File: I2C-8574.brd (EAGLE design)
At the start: 106 x 100 mm, 89 parts, among them J1 CONNECTOR-I2CLEFT, J11 RJ12/6, J2 CONNECTOR-I2CLEFT, J5 CONNECTOR-GROVE-4P-2.0-347013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, J6 RJ12/6, J7 RJ12/6, J8 CONNECTOR-GROVE-4P-2.0-347013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, J9 RJ12/6, U1 PCF8574DW, U2 PCF8574ADW

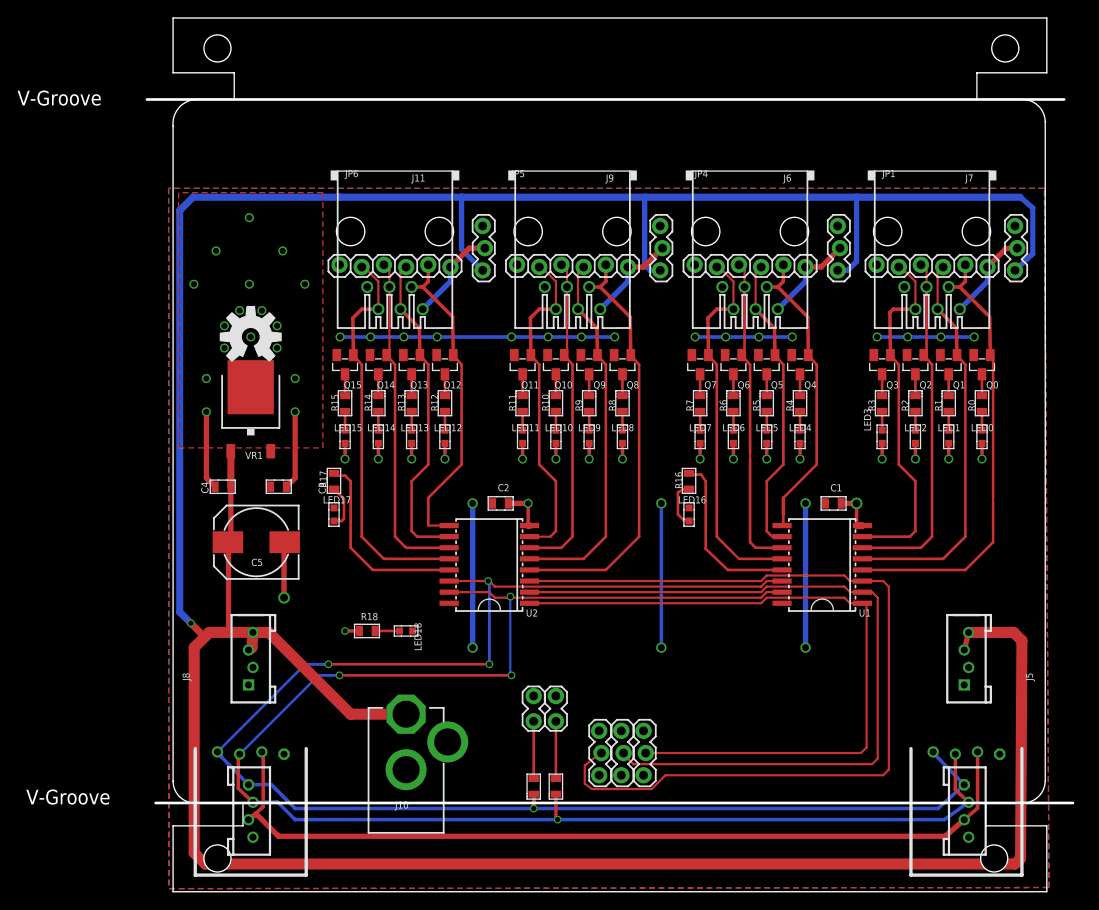
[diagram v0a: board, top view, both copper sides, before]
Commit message: 3.0
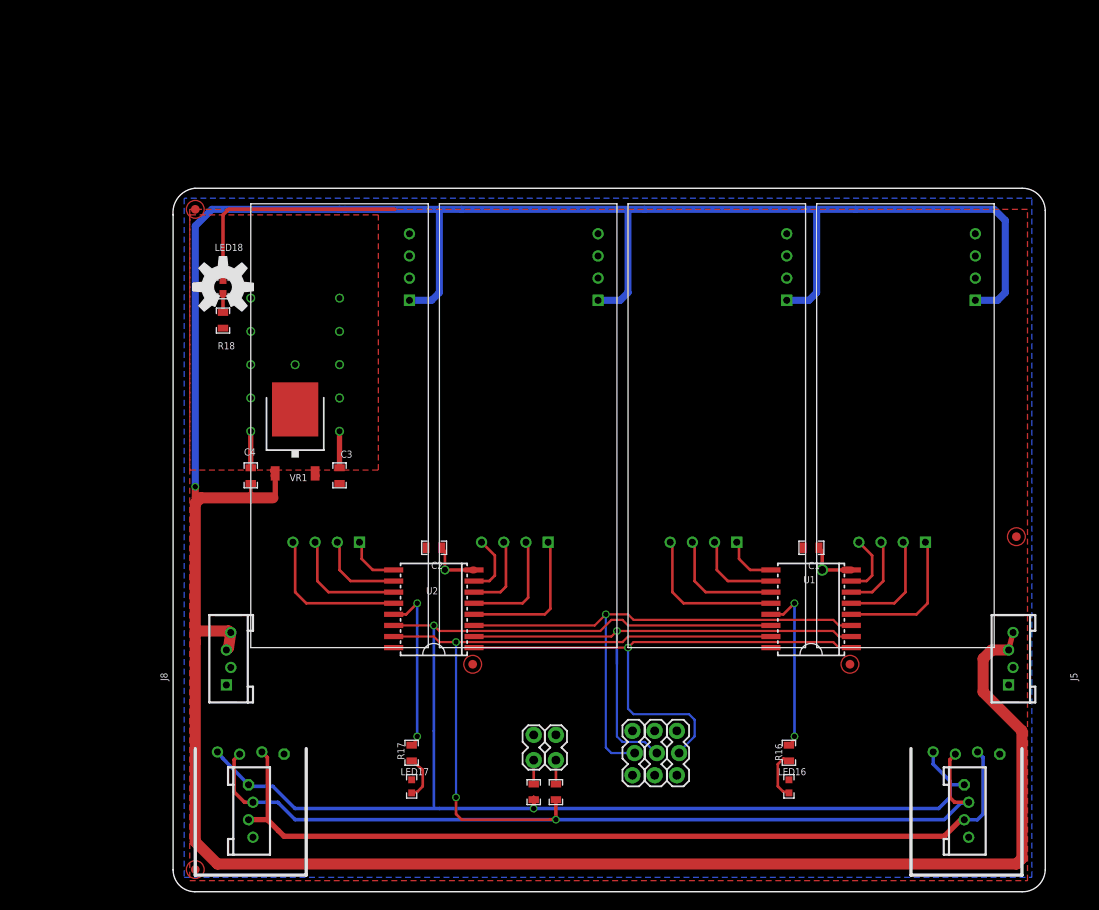
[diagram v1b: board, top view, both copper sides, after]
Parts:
- removed C5: 150uF, SPCoast:0810-CAP
- removed J10: (no value), SPCoast:DCJ0202
- removed J11, J6, J7, J9: RJ12/6, SPCoast:RJ25-PANEL
- removed JP1, JP4, JP5, JP6: .100x1x6, SPCoast:1X06_LOCK
- removed LED0, LED1, LED10, LED11, LED12, LED13, LED14, LED15, LED2, LED3, LED4, LED5, LED6, LED7, LED8, LED9: Y-0330050P1, SPCoast:0603-LED
- removed POWER: 7-12vDC, SPCoast-minimal:POWER_USAGE
- removed Q0, Q1, Q10, Q11, Q12, Q13, Q14, Q15, Q2, Q3, Q4, Q5, Q6, Q7, Q8, Q9: (no value), SPCoast:SOT23
- removed R0, R1, R10, R11, R12, R13, R14, R2, R3, R4, R5, R6, R7, R8, R9: 2K2, SPCoast:0805-RES
- removed R15: 2K0, SPCoast:0805-RES
- removed VIO1, VIO2, VIO3, VIO4: jumper, SPCoast:1X03
- added FID-U1, FID-U2, FID1, FID2, FID3: FIDUCIAL, SPCoast:FIDUCIAL_1MM
- added U$2, U$3, U$4, U$5: IO4-IOBBARE, SPCoast:IO4-IOB
- A1, A2, A3: device SPCoast:1X03 -> SPCoast-minimal:1X03
- BOARD1: value BOARD80X100-NOHOLES -> (none)
- C1, C2, C3, C4: device SPCoast:0805-CAP -> SPCoast-minimal:0805-CAP
- R16, R17, R18: device SPCoast:0805-RES -> SPCoast-minimal:0805-RES
- SCL, SDA: device SPCoast:1X02_LOCK -> SPCoast-minimal:1X02_LOCK
- U1, U2: device SPCoast:SO-16DW -> SPCoast-minimal:SO-16DW
- moved LED18 44.6 mm to (5.71, 69.2), turned to 270 degrees
- moved R18 39.2 mm to (5.71, 65.4), turned to 270 degrees
- moved LED16 33.1 mm to (70.5, 12.1)
- moved R16 33.1 mm to (70.5, 15.9)
- moved LED17 32.4 mm to (27.3, 12.1)
- moved R17 32.4 mm to (27.3, 15.9)
- moved C2 9.16 mm to (29.8, 39.4)
- moved U2 8.13 mm to (29.8, 32.4)
- moved C3 7.10 mm to (19.1, 47.6), turned to 90 degrees
- moved U$1 6.54 mm to (5.71, 69.2)
- moved C1 5.68 mm to (73.0, 39.4)
- moved VR1 5.68 mm to (14.0, 52.7)
- moved U1 5.24 mm to (73.0, 32.4)
- moved J5 5.08 mm to (95.9, 26.7)
- moved SCL 4.44 mm to (43.8, 15.2)
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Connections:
- removed net N$10: LED7.A, R7.1
- removed net N$11: Q0.3, R0.2
- removed net N$12: Q5.3, R5.2
- removed net N$13: Q6.3, R6.2
- removed net N$14: Q7.3, R7.2
- removed net N$15: LED8.A, R8.1
- removed net N$16: LED9.A, R9.1
- removed net N$17: LED10.A, R10.1
- removed net N$18: Q8.3, R8.2
- removed net N$2: LED0.A, R0.1
- removed net N$22: Q9.3, R9.2
- removed net N$23: Q10.3, R10.2
- removed net N$24: Q11.3, R11.2
- removed net N$25: LED11.A, R11.1
- removed net N$26: LED14.A, R14.1
- removed net N$27: LED12.A, R12.1
- removed net N$28: LED13.A, R13.1
- removed net N$29: LED15.A, R15.1
- removed net N$3: LED1.A, R1.1
- removed net N$30: Q1.3, R1.2
- removed net N$31: Q2.3, R2.2
- removed net N$32: Q3.3, R3.2
- removed net N$33: Q12.3, R12.2
- removed net N$34: Q13.3, R13.2
- removed net N$35: Q14.3, R14.2
- removed net N$36: Q15.3, R15.2
- removed net N$4: LED2.A, R2.1
- removed net N$5: LED3.A, R3.1
- removed net N$6: LED4.A, R4.1
- removed net N$7: LED5.A, R5.1
- removed net N$8: Q4.3, R4.2
- removed net N$9: LED6.A, R6.1
- removed net VCC-IO1: J7.1, JP1.6, VIO1.2
- removed net VCC-IO2: J6.1, JP4.6, VIO2.2
- removed net VCC-IO3: J9.1, JP5.6, VIO3.2
- removed net VCC-IO4: J11.1, JP6.6, VIO4.2
- net +9V: now also U$2.V+, U$3.V+, U$4.V+, U$5.V+; no longer C5.+, J10.1, VIO1.3, VIO2.3, VIO3.3, VIO4.3
- net GND: now also U$2.G@1, U$2.G@2, U$3.G@1, U$3.G@2, U$4.G@1, U$4.G@2, U$5.G@1, U$5.G@2; no longer C5.-, J10.2, J10.3, J11.6, J6.6, J7.6, J9.6, JP1.1, JP4.1, JP5.1, JP6.1, LED0.C, LED1.C, LED10.C, LED11.C, LED12.C, LED13.C, LED14.C, LED15.C, LED2.C, LED3.C, LED4.C, LED5.C, LED6.C, LED7.C, LED8.C, LED9.C
- net P1: now also U$2.P1; no longer J7.2, JP1.5, Q0.1
- net P10: now also U$4.P2; no longer J9.3, JP5.4, Q9.1
- net P11: now also U$4.P3; no longer J9.4, JP5.3, Q10.1
- net P12: now also U$4.P4; no longer J9.5, JP5.2, Q11.1
- net P13: now also U$5.P1; no longer J11.2, JP6.5, Q12.1
- net P14: now also U$5.P2; no longer J11.3, JP6.4, Q13.1
- net P15: now also U$5.P3; no longer J11.4, JP6.3, Q14.1
- net P16: now also U$5.P4; no longer J11.5, JP6.2, Q15.1
- net P2: now also U$2.P2; no longer J7.3, JP1.4, Q1.1
- net P3: now also U$2.P3; no longer J7.4, JP1.3, Q2.1
- net P4: now also U$2.P4; no longer J7.5, JP1.2, Q3.1
- net P5: now also U$3.P1; no longer J6.2, JP4.5, Q4.1
- net P6: now also U$3.P2; no longer J6.3, JP4.4, Q5.1
- net P7: now also U$3.P3; no longer J6.4, JP4.3, Q6.1
- net P8: now also U$3.P4; no longer J6.5, JP4.2, Q7.1
- net P9: now also U$4.P1; no longer J9.2, JP5.5, Q8.1
- net VCC: now also U$2.V5, U$3.V5, U$4.V5, U$5.V5; no longer Q0.2, Q1.2, Q10.2, Q11.2, Q12.2, Q13.2, Q14.2, Q15.2, Q2.2, Q3.2, Q4.2, Q5.2, Q6.2, Q7.2, Q8.2, Q9.2, VIO1.1, VIO2.1, VIO3.1, VIO4.1
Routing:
- net VCC: track 103.3 -> 27.9 mm, vias 22 -> 0
- net GND: track 65.4 -> 20.4 mm, vias 37 -> 13
- net A2: track 103.3 -> 63.0 mm, vias 0 -> 1
- net P1: track 51.1 -> 16.4 mm
- net P4: track 41.4 -> 7.09 mm
- net P2: track 45.2 -> 12.5 mm
- net P9: track 48.5 -> 16.7 mm
- net P3: track 40.4 -> 8.73 mm
- net P13: track 37.1 -> 6.19 mm
- net P12: track 37.9 -> 7.09 mm
- net P10: track 42.2 -> 12.9 mm
- net P5: track 34.9 -> 6.19 mm
- net P11: track 37.3 -> 9.10 mm
- net P16: track 45.5 -> 17.6 mm
- net P14: track 37.1 -> 10.0 mm
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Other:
- board size 106 x 100 mm -> 99.8 x 80.5 mm
- board text added: "'74A"
- board text added: "16 bit I2C Digital I/O Active Low"
- board text added: "2017.10"
- board text added: "4 3 2 1"
- board text added: "8 7 6 5"
- board text added: "External daughterboards for each IO bank Eliminates having to custom cut 3M track Eliminates having to stock signal driver I2C boards Custom input low pass filters can be added to Detector and Turtle drivers"
- board text added: "I/O lines"
- board text added: "Input Changed"
- board text added: "gnd"
- board text added: "v3.0"
- board text removed: "- 4 3 2 1 +"
- board text removed: "- 8 7 6 5 +"
- board text removed: "1.5A"
- board text removed: "16 bit I2C Digital I/O with visual feedback"
- board text removed: "2014.04"
- board text removed: "2014.07"
- board text removed: "2014.10"
- board text removed: "2016.10"
- board text removed: "2017.07"
- board text removed: "2k0"
- board text removed: "A"
- board text removed: "Do Not Populate 6x1 0.100 hdrs"
- board text removed: "Green"
- board text removed: "Green (3 places)"
- board text removed: "IO4"
- board text removed: "Note: IC on left has "A" suffix, IC on right does not!"
- board text removed: "P-FET"
- board text removed: "Power"
- board text removed: "Vio for each port selectable between 5V and VIN"
- board text removed: "Yellow"
- board text removed: "v2.4"
